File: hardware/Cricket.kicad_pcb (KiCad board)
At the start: 2 copper layers, 67.5 x 38.5 mm, 14 parts, among them J1 S2B-XH-A, Q1 RQ6C065BCTCR, SW1 SW_SPDT, U1 Seeed Xiao ESP32C3, U2 DFR0299

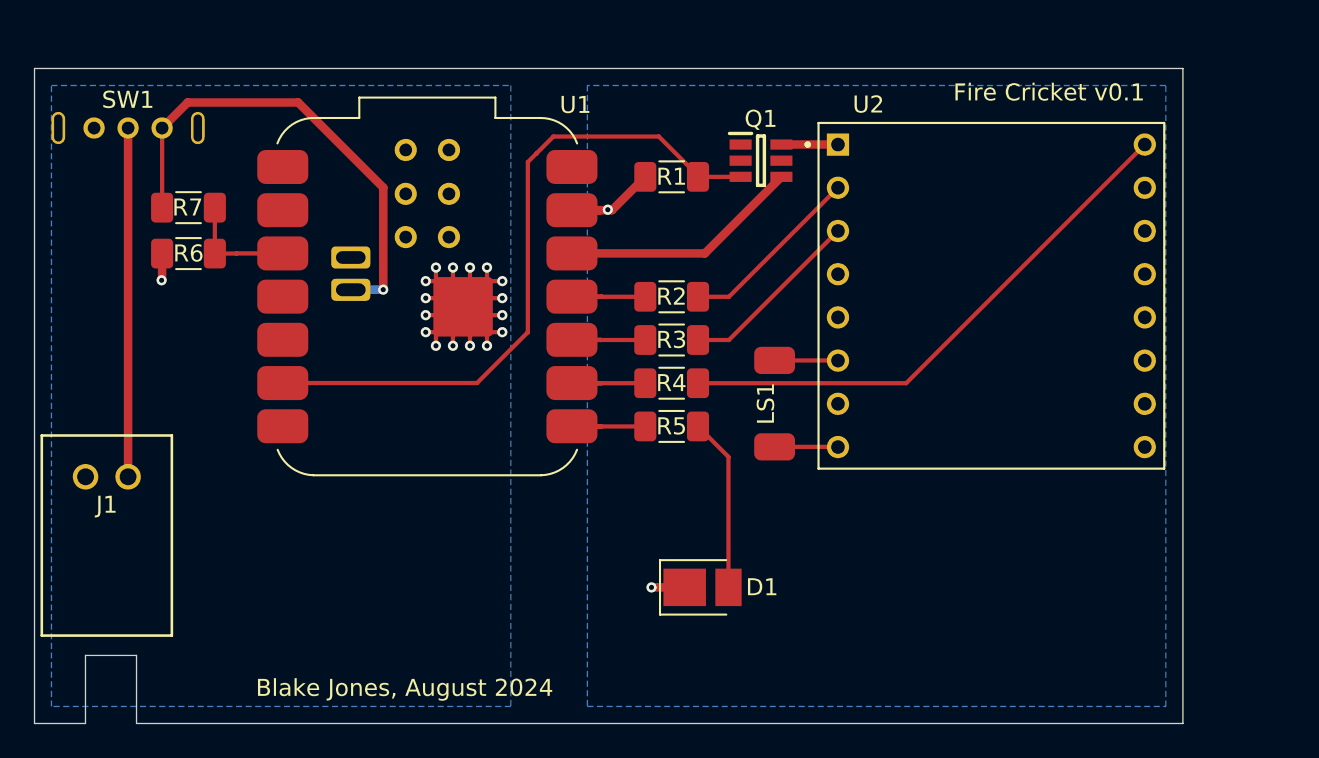
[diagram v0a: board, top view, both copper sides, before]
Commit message: v0.2 tapeout
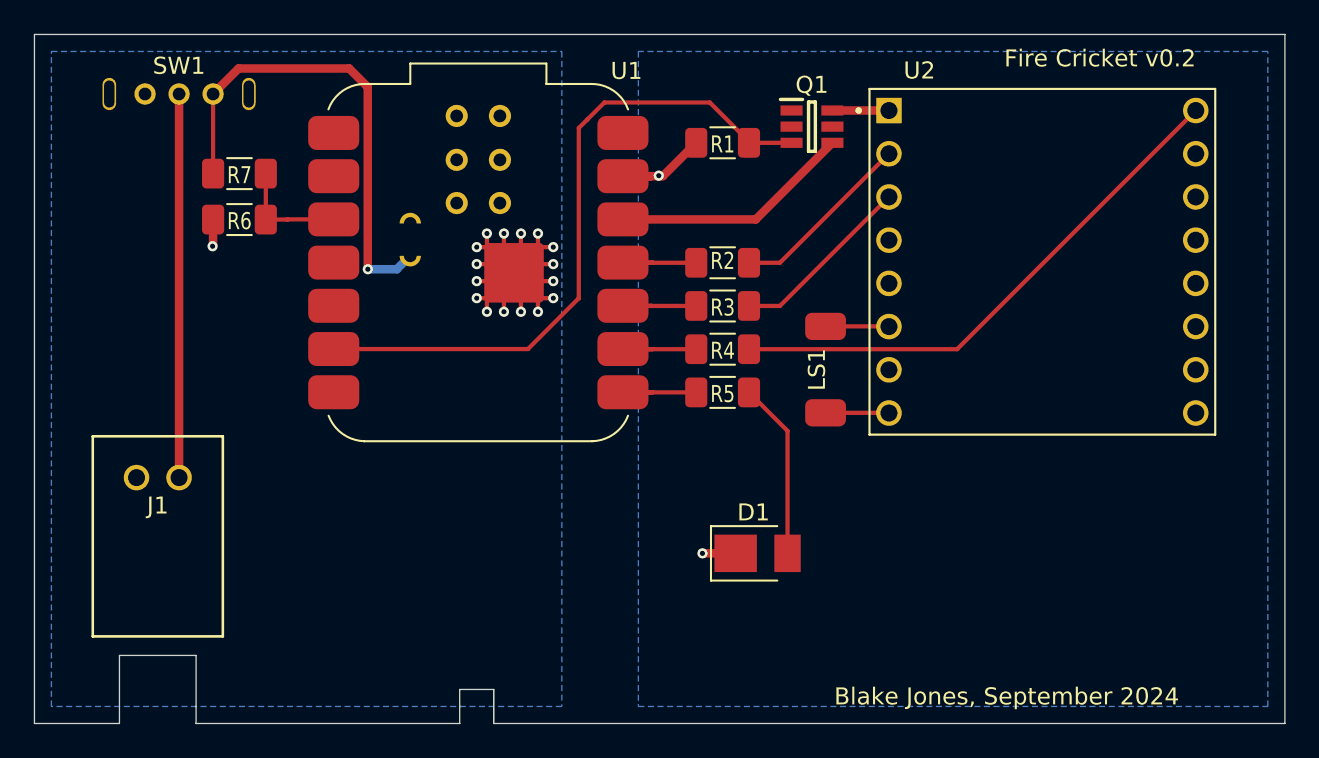
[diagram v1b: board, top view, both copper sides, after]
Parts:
- D1: footprint LED_SMD:LED_PLCC_2835_Handsoldering -> Cricket_footprints:LED_PLCC_2835
- R1, R2, R3, R4, R5, R6, R7: footprint Resistor_SMD:R_1206_3216Metric_Pad1.30x1.75mm_HandSolder -> Cricket_footprints:R_1206_3216Metric_Pad1.30x1.75mm_HandSolder
- U1: footprint RF_Module:MCU_Seeed_ESP32C3 -> Cricket_footprints:Seeed_Xiao_ESP32C3
- moved LS1 3.60 mm to (146.5, 79.2)
- moved U1 3.60 mm to (126.1, 72.9)
- moved R6 3.60 mm to (112.0, 70.4)
- moved R7 3.60 mm to (112.0, 67.7)
- moved SW1 3.60 mm to (108.5, 63.0)
- moved D1 3.60 mm to (142.3, 90.0)
- moved Q1 3.60 mm to (145.7, 64.9)
- moved R1 3.60 mm to (140.4, 65.9)
- moved R2 3.60 mm to (140.4, 72.9)
- moved R3 3.60 mm to (140.4, 75.5)
- moved R4 3.60 mm to (140.4, 78.0)
- moved R5 3.60 mm to (140.4, 80.5)
- moved U2 3.60 mm to (159.2, 72.9)
- moved J1 3.00 mm to (106.0, 85.5)
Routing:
- net VCC: track 20.5 -> 22.5 mm
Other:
- board size 67.5 x 38.5 mm -> 73.5 x 40.5 mm
- board text added: "Blake Jones, September 2024"
- board text added: "Fire Cricket v0.2"
- board text removed: "Blake Jones, August 2024"
- board text removed: "Fire Cricket v0.1"

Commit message: Hardware for v0.2a (PCBA)
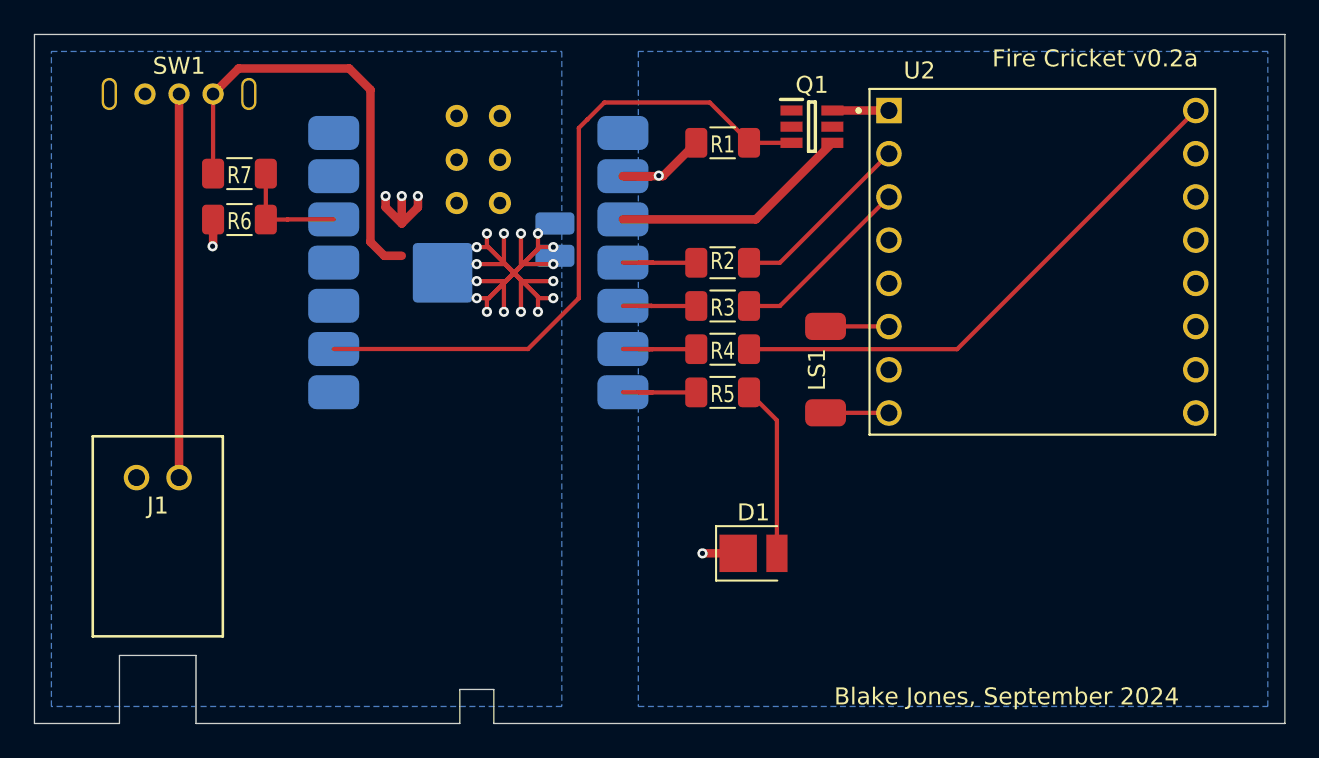
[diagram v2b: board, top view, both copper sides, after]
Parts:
- D1: footprint Cricket_footprints:LED_PLCC_2835 -> LED_SMD:LED_PLCC_2835
- U1: footprint Cricket_footprints:Seeed_Xiao_ESP32C3 -> RF_Module:MCU_Seeed_ESP32C3; moved to B.Cu
- turned U1 to 180 degrees
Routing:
- net GND: track 44.6 -> 50.2 mm, vias 17 -> 20
- net Net-(SW1-C): track 28.4 -> 26.2 mm, vias 1 -> 0
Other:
- board text added: "Fire Cricket v0.2a"
- board text removed: "Fire Cricket v0.2"
